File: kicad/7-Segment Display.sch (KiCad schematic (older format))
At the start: 23 parts, among them U7 74AC574, U8 74AC574, U9 74AHC02

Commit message: Working on SD card interface, cleaning up.
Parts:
- removed U7, U8: 74AC574, Housings_DIP:DIP-20_W7.62mm_LongPads, symbol 74xx:74LS574
- added U7, U8: 74AC273, symbol 74xx:74LS273
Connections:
- net labels added: ~RESET
- wire segments 77 -> 79
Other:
- moved on the sheet: R21, R22, R23, R24, R25, R26, R27, R28
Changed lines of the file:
@@
 $Descr USLetter 11000 8500
 encoding utf-8
-Sheet 3 9
+Sheet 3 10
 Title "7-Segment Display"
 Date "2018-07-20"
@@
 Comment4 ""
 $EndDescr
-$Comp
-L power:GND #PWR032
-U 1 1 59D6D694
-P 4950 4000
-F 0 "#PWR032" H 4950 3750 50  0001 C CNN
-F 1 "GND" H 4950 3850 50  0000 C CNN
-F 2 "" H 4950 4000 50  0001 C CNN
-F 3 "" H 4950 4000 50  0001 C CNN
-	1    4950 4000
-	1    0    0    -1
-$EndComp
 Entry Wire Line
 	4500 3500 4600 3400
@@
 D7
 $Comp
-L 74xx:74LS574 U7
-U 1 1 59D6D6AA
-P 5450 3200
-F 0 "U7" H 5450 3200 50  0000 C CNN
-F 1 "74AC574" H 5500 2850 50  0000 C CNN
-F 2 "Housings_DIP:DIP-20_W7.62mm_LongPads" H 5450 3200 50  0001 C CNN
-F 3 "" H 5450 3200 50  0001 C CNN
-	1    5450 3200
-	1    0    0    -1
-$EndComp
-$Comp
 L Device:R R12
 U 1 1 59D6D6B1
@@
 	0    1    1    0
 $EndComp
-$Comp
-L power:GND #PWR033
-U 1 1 59D6D6E9
-P 4950 5550
-F 0 "#PWR033" H 4950 5300 50  0001 C CNN
-F 1 "GND" H 4950 5400 50  0000 C CNN
-F 2 "" H 4950 5550 50  0001 C CNN
-F 3 "" H 4950 5550 50  0001 C CNN
-	1    4950 5550
-	1    0    0    -1
-$EndComp
+Entry Wire Line
+	4500 5550 4600 5450
+Entry Wire Line
+	4500 5450 4600 5350
 Entry Wire Line
 	4500 5350 4600 5250
@@
 Entry Wire Line
 	4500 4850 4600 4750
-Entry Wire Line
-	4500 4750 4600 4650
-Entry Wire Line
-	4500 4650 4600 4550
-Text Label 4600 4550 0    60   ~ 0
+Text Label 4600 4750 0    60   ~ 0
 D0
-Text Label 4600 4650 0    60   ~ 0
+Text Label 4600 4850 0    60   ~ 0
 D1
-Text Label 4600 4750 0    60   ~ 0
+Text Label 4600 4950 0    60   ~ 0
 D2
-Text Label 4600 4850 0    60   ~ 0
+Text Label 4600 5050 0    60   ~ 0
 D3
-Text Label 4600 4950 0    60   ~ 0
+Text Label 4600 5150 0    60   ~ 0
 D4
-Text Label 4600 5050 0    60   ~ 0
+Text Label 4600 5250 0    60   ~ 0
 D5
-Text Label 4600 5150 0    60   ~ 0
+Text Label 4600 5350 0    60   ~ 0
 D6
-Text Label 4600 5250 0    60   ~ 0
+Text Label 4600 5450 0    60   ~ 0
 D7
-$Comp
-L 74xx:74LS574 U8
-U 1 1 59D6D6FF
-P 5450 5050
-F 0 "U8" H 5450 5050 50  0000 C CNN
-F 1 "74AC574" H 5500 4700 50  0000 C CNN
-F 2 "Housings_DIP:DIP-20_W7.62mm_LongPads" H 5450 5050 50  0001 C CNN
-F 3 "" H 5450 5050 50  0001 C CNN
-	1    5450 5050
-	1    0    0    -1
-$EndComp
 $Comp
 L Device:R R21
 U 1 1 59D6D706
-P 6300 4550
-F 0 "R21" V 6261 4660 50  0000 L CNN
-F 1 "220R" V 6300 4550 50  0000 C CNN
-F 2 "Resistors_THT:R_Axial_DIN0204_L3.6mm_D1.6mm_P5.08mm_Horizontal" V 6230 4550 50  0001 C CNN
-F 3 "" H 6300 4550 50  0001 C CNN
-	1    6300 4550
-	0    1    1    0
-$EndComp
-$Comp
-L Device:R R22
-U 1 1 59D6D70D
-P 6300 4650
-F 0 "R22" V 6261 4760 50  0000 L CNN
-F 1 "220R" V 6300 4650 50  0000 C CNN
-F 2 "Resistors_THT:R_Axial_DIN0204_L3.6mm_D1.6mm_P5.08mm_Horizontal" V 6230 4650 50  0001 C CNN
-F 3 "" H 6300 4650 50  0001 C CNN
-	1    6300 4650
-	0    1    1    0
-$EndComp
-$Comp
-L Device:R R23
-U 1 1 59D6D714
 P 6300 4750
-F 0 "R23" V 6261 4860 50  0000 L CNN
+F 0 "R21" V 6261 4860 50  0000 L CNN
 F 1 "220R" V 6300 4750 50  0000 C CNN
 F 2 "Resistors_THT:R_Axial_DIN0204_L3.6mm_D1.6mm_P5.08mm_Horizontal" V 6230 4750 50  0001 C CNN
@@
 $EndComp
 $Comp
-L Device:R R24
-U 1 1 59D6D71B
+L Device:R R22
+U 1 1 59D6D70D
 P 6300 4850
-F 0 "R24" V 6261 4960 50  0000 L CNN
+F 0 "R22" V 6261 4960 50  0000 L CNN
 F 1 "220R" V 6300 4850 50  0000 C CNN
 F 2 "Resistors_THT:R_Axial_DIN0204_L3.6mm_D1.6mm_P5.08mm_Horizontal" V 6230 4850 50  0001 C CNN
@@
 $EndComp
 $Comp
-L Device:R R25
-U 1 1 59D6D722
+L Device:R R23
+U 1 1 59D6D714
 P 6300 4950
-F 0 "R25" V 6261 5060 50  0000 L CNN
+F 0 "R23" V 6261 5060 50  0000 L CNN
 F 1 "220R" V 6300 4950 50  0000 C CNN
 F 2 "Resistors_THT:R_Axial_DIN0204_L3.6mm_D1.6mm_P5.08mm_Horizontal" V 6230 4950 50  0001 C CNN
@@
 $EndComp
 $Comp
-L Device:R R26
-U 1 1 59D6D729
+L Device:R R24
+U 1 1 59D6D71B
 P 6300 5050
-F 0 "R26" V 6261 5160 50  0000 L CNN
+F 0 "R24" V 6261 5160 50  0000 L CNN
 F 1 "220R" V 6300 5050 50  0000 C CNN
 F 2 "Resistors_THT:R_Axial_DIN0204_L3.6mm_D1.6mm_P5.08mm_Horizontal" V 6230 5050 50  0001 C CNN
@@
 $EndComp
 $Comp
-L Device:R R27
-U 1 1 59D6D730
+L Device:R R25
+U 1 1 59D6D722
 P 6300 5150
-F 0 "R27" V 6261 5260 50  0000 L CNN
+F 0 "R25" V 6261 5260 50  0000 L CNN
 F 1 "220R" V 6300 5150 50  0000 C CNN
 F 2 "Resistors_THT:R_Axial_DIN0204_L3.6mm_D1.6mm_P5.08mm_Horizontal" V 6230 5150 50  0001 C CNN
@@
 $EndComp
 $Comp
-L Device:R R28
-U 1 1 59D6D737
+L Device:R R26
+U 1 1 59D6D729
 P 6300 5250
-F 0 "R28" V 6261 5360 50  0000 L CNN
+F 0 "R26" V 6261 5360 50  0000 L CNN
 F 1 "220R" V 6300 5250 50  0000 C CNN
 F 2 "Resistors_THT:R_Axial_DIN0204_L3.6mm_D1.6mm_P5.08mm_Horizontal" V 6230 5250 50  0001 C CNN
 F 3 "" H 6300 5250 50  0001 C CNN
 	1    6300 5250
+	0    1    1    0
+$EndComp
+$Comp
+L Device:R R27
+U 1 1 59D6D730
+P 6300 5350
+F 0 "R27" V 6261 5460 50  0000 L CNN
+F 1 "220R" V 6300 5350 50  0000 C CNN
+F 2 "Resistors_THT:R_Axial_DIN0204_L3.6mm_D1.6mm_P5.08mm_Horizontal" V 6230 5350 50  0001 C CNN
+F 3 "" H 6300 5350 50  0001 C CNN
+	1    6300 5350
+	0    1    1    0
+$EndComp
+$Comp
+L Device:R R28
+U 1 1 59D6D737
+P 6300 5450
+F 0 "R28" V 6261 5560 50  0000 L CNN
+F 1 "220R" V 6300 5450 50  0000 C CNN
+F 2 "Resistors_THT:R_Axial_DIN0204_L3.6mm_D1.6mm_P5.08mm_Horizontal" V 6230 5450 50  0001 C CNN
+F 3 "" H 6300 5450 50  0001 C CNN
+	1    6300 5450
 	0    1    1    0
 $EndComp
@@
 	8200 2700 8250 2700
 Wire Wire Line
-	8250 4550 6450 4550
+	8250 4750 6450 4750
 Wire Wire Line
 	8200 2800 8300 2800
 Wire Wire Line
-	8300 4650 6450 4650
+	8300 4850 6450 4850
 Wire Wire Line
 	8200 2900 8350 2900
 Wire Wire Line
-	8350 4750 6450 4750
+	8350 4950 6450 4950
 Wire Wire Line
 	8200 3000 8400 3000
 Wire Wire Line
-	8400 4850 6450 4850
+	8400 5050 6450 5050
 Wire Wire Line
 	8200 3100 8450 3100
 Wire Wire Line
-	8450 4950 6450 4950
+	8450 5150 6450 5150
 Wire Wire Line
 	8200 3200 8500 3200
 Wire Wire Line
-	8500 5050 6450 5050
+	8500 5250 6450 5250
 Wire Wire Line
 	8200 3300 8550 3300
 Wire Wire Line
-	8550 5150 6450 5150
+	8550 5350 6450 5350
 Wire Wire Line
 	8200 3400 8600 3400
 Wire Wire Line
-	8600 5250 6450 5250
+	8600 5450 6450 5450
 $Comp
 L power:GND #PWR034
@@
 Wire Wire Line
 	1450 5000 3200 5000
-Text HLabel 1450 2250 0    60   BiDi ~ 0
+Text HLabel 1450 2450 0    60   BiDi ~ 0
 D[0..7]
 Wire Bus Line
-	1450 2250 4500 2250
+	1450 2450 4500 2450
 Text HLabel 1450 3500 0    60   Input ~ 0
 ~WR
@@
 	3800 3600 4950 3600
 Wire Wire Line
-	4600 4550 4950 4550
-Wire Wire Line
-	4600 4650 4950 4650
-Wire Wire Line
 	4600 4750 4950 4750
 Wire Wire Line
@@
 	4600 5250 4950 5250
 Wire Wire Line
-	3800 5450 4950 5450
-Wire Wire Line
-	5950 4550 6150 4550
-Wire Wire Line
-	6150 4650 5950 4650
+	4600 5350 4950 5350
+Wire Wire Line
+	4600 5450 4950 5450
+Wire Wire Line
+	3800 5650 4950 5650
 Wire Wire Line
 	5950 4750 6150 4750
@@
 Wire Wire Line
 	6150 5250 5950 5250
+Wire Wire Line
+	5950 5350 6150 5350
+Wire Wire Line
+	6150 5450 5950 5450
 Wire Wire Line
 	5950 2700 6150 2700
@@
 L power:GND #PWR0108
 U 1 1 5C4980BE
-P 5450 5850
-F 0 "#PWR0108" H 5450 5600 50  0001 C CNN
-F 1 "GND" H 5455 5677 50  0000 C CNN
-F 2 "" H 5450 5850 50  0001 C CNN
-F 3 "" H 5450 5850 50  0001 C CNN
-	1    5450 5850
-	1    0    0    -1
-$EndComp
-Wire Wire Line
-	5450 4000 4950 4000
-Wire Wire Line
-	4950 4000 4950 3700
+P 5450 6050
+F 0 "#PWR0108" H 5450 5800 50  0001 C CNN
+F 1 "GND" H 5455 5877 50  0000 C CNN
+F 2 "" H 5450 6050 50  0001 C CNN
+F 3 "" H 5450 6050 50  0001 C CNN
+	1    5450 6050
+	1    0    0    -1
+$EndComp
 $Comp
 L power:VCC #PWR0109
 U 1 1 5C4A51B5
-P 5450 4250
-F 0 "#PWR0109" H 5450 4100 50  0001 C CNN
-F 1 "VCC" H 5467 4423 50  0000 C CNN
-F 2 "" H 5450 4250 50  0001 C CNN
-F 3 "" H 5450 4250 50  0001 C CNN
-	1    5450 4250
-	1    0    0    -1
-$EndComp
-Wire Wire Line
-	3800 5450 3800 4900
-Wire Wire Line
-	8250 2700 8250 4550
-Wire Wire Line
-	8300 2800 8300 4650
-Wire Wire Line
-	8350 2900 8350 4750
-Wire Wire Line
-	8400 3000 8400 4850
-Wire Wire Line
-	8450 3100 8450 4950
-Wire Wire Line
-	8500 3200 8500 5050
-Wire Wire Line
-	8550 3300 8550 5150
-Wire Wire Line
-	8600 3400 8600 5250
+P 5450 4450
+F 0 "#PWR0109" H 5450 4300 50  0001 C CNN
+F 1 "VCC" H 5467 4623 50  0000 C CNN
+F 2 "" H 5450 4450 50  0001 C CNN
+F 3 "" H 5450 4450 50  0001 C CNN
+	1    5450 4450
+	1    0    0    -1
+$EndComp
+$Comp
+L 74xx:74LS273 U7
+U 1 1 5C73DF7A
+P 5450 3200
+F 0 "U7" H 5200 3850 50  0000 C CNN
+F 1 "74AC273" H 5650 2550 50  0000 C CNN
+F 2 "" H 5450 3200 50  0001 C CNN
+F 3 "http://www.ti.com/lit/gpn/sn74LS273" H 5450 3200 50  0001 C CNN
+	1    5450 3200
+	1    0    0    -1
+$EndComp
+$Comp
+L 74xx:74LS273 U8
+U 1 1 5C74152B
+P 5450 5250
+F 0 "U8" H 5200 5900 50  0000 C CNN
+F 1 "74AC273" H 5650 4600 50  0000 C CNN
+F 2 "" H 5450 5250 50  0001 C CNN
+F 3 "http://www.ti.com/lit/gpn/sn74LS273" H 5450 5250 50  0001 C CNN
+	1    5450 5250
+	1    0    0    -1
+$EndComp
+$Comp
+L power:GND #PWR?
+U 1 1 5C74297B
+P 5450 4000
+F 0 "#PWR?" H 5450 3750 50  0001 C CNN
+F 1 "GND" H 5455 3827 50  0000 C CNN
+F 2 "" H 5450 4000 50  0001 C CNN
+F 3 "" H 5450 4000 50  0001 C CNN
+	1    5450 4000
+	1    0    0    -1
+$EndComp
+Wire Wire Line
+	3800 4900 3800 5650
+Wire Wire Line
+	8250 2700 8250 4750
+Wire Wire Line
+	8300 2800 8300 4850
+Wire Wire Line
+	8350 2900 8350 4950
+Wire Wire Line
+	8400 3000 8400 5050
+Wire Wire Line
+	8450 3100 8450 5150
+Wire Wire Line
+	8500 3200 8500 5250
+Wire Wire Line
+	8550 3300 8550 5350
+Wire Wire Line
+	8600 3400 8600 5450
+Text HLabel 1450 5750 0    60   Input ~ 0
+~RESET
+Wire Wire Line
+	1450 5750 4350 5750
+Wire Wire Line
+	4950 3700 4350 3700
+Wire Wire Line
+	4350 3700 4350 5750
 Wire Bus Line
-	4500 2250 4500 5350
-Connection ~ 4950 4000
+	4500 2450 4500 5550
+Connection ~ 4350 5750
+Wire Wire Line
+	4350 5750 4950 5750
 $EndSCHEMATC

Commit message: Assign footprints.
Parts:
- U7, U8: footprint (none) -> Housings_SSOP:TSSOP-20_4.4x6.5mm_Pitch0.65mm
- U9: footprint Housings_DIP:DIP-14_W7.62mm_LongPads -> Housings_DIP:DIP-14_W7.62mm
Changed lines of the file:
@@
 F 0 "U9" H 3500 3650 50  0000 C CNN
 F 1 "74AHC02" H 3550 3550 50  0000 C CNN
-F 2 "Housings_DIP:DIP-14_W7.62mm_LongPads" H 3500 3600 50  0001 C CNN
+F 2 "Housings_DIP:DIP-14_W7.62mm" H 3500 3600 50  0001 C CNN
 F 3 "" H 3500 3600 50  0001 C CNN
 	1    3500 3600
@@
 F 0 "U9" H 3500 4950 50  0000 C CNN
 F 1 "74AHC02" H 3550 4850 50  0000 C CNN
-F 2 "Housings_DIP:DIP-14_W7.62mm_LongPads" H 3500 4900 50  0001 C CNN
+F 2 "Housings_DIP:DIP-14_W7.62mm" H 3500 4900 50  0001 C CNN
 F 3 "" H 3500 4900 50  0001 C CNN
 	2    3500 4900
@@
 F 0 "U7" H 5200 3850 50  0000 C CNN
 F 1 "74AC273" H 5650 2550 50  0000 C CNN
-F 2 "" H 5450 3200 50  0001 C CNN
+F 2 "Housings_SSOP:TSSOP-20_4.4x6.5mm_Pitch0.65mm" H 5450 3200 50  0001 C CNN
 F 3 "http://www.ti.com/lit/gpn/sn74LS273" H 5450 3200 50  0001 C CNN
 	1    5450 3200
@@
 F 0 "U8" H 5200 5900 50  0000 C CNN
 F 1 "74AC273" H 5650 4600 50  0000 C CNN
-F 2 "" H 5450 5250 50  0001 C CNN
+F 2 "Housings_SSOP:TSSOP-20_4.4x6.5mm_Pitch0.65mm" H 5450 5250 50  0001 C CNN
 F 3 "http://www.ti.com/lit/gpn/sn74LS273" H 5450 5250 50  0001 C CNN
 	1    5450 5250

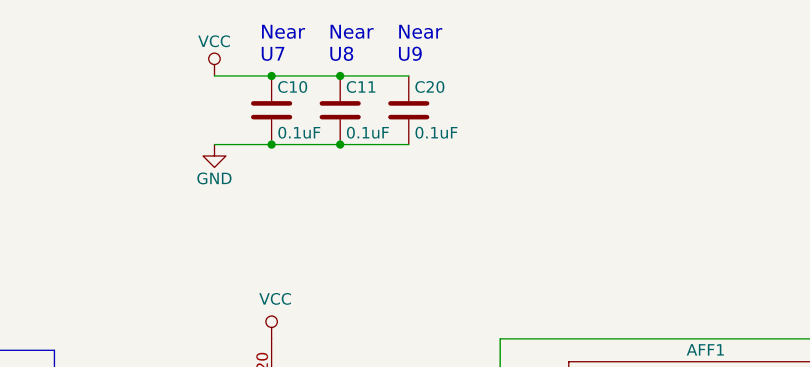
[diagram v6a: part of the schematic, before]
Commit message: First pass layout of revised board complete.
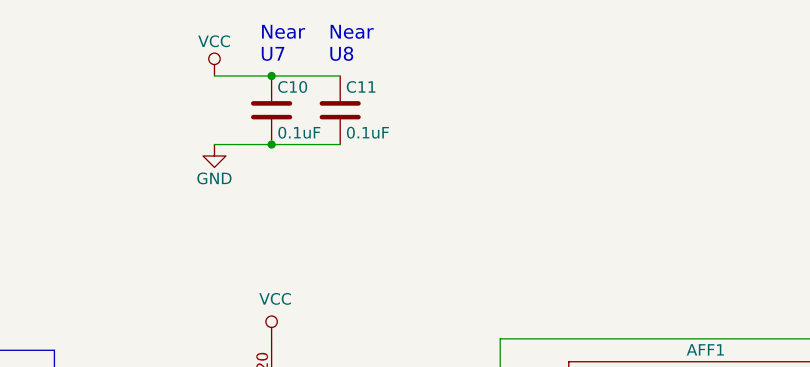
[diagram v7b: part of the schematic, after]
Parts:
- removed C20: 0.1uF, Capacitors_THT:C_Disc_D4.3mm_W1.9mm_P5.00mm, symbol Device:C
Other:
- note removed: "Near\nU9"
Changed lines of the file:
@@
 Sheet 3 11
 Title "7-Segment Display"
-Date "2019-04-11"
+Date "2019-04-15"
 Rev "1"
 Comp ""
@@
 Connection ~ 5450 1250
 Connection ~ 5450 1550
-Connection ~ 5750 1250
-Connection ~ 5750 1550
 Wire Wire Line
 	5200 1550 5450 1550
@@
 	1    0    0    -1
 $EndComp
-$Comp
-L Device:C C20
-U 1 1 59EFD5EA
-P 6050 1400
-F 0 "C20" H 6075 1500 50  0000 L CNN
-F 1 "0.1uF" H 6075 1300 50  0000 L CNN
-F 2 "Capacitors_THT:C_Disc_D4.3mm_W1.9mm_P5.00mm" H 6088 1250 50  0001 C CNN
-F 3 "" H 6050 1400 50  0001 C CNN
-	1    6050 1400
-	1    0    0    -1
-$EndComp
-Text Notes 6000 1200 0    60   ~ 0
-Near\nU9
 Wire Wire Line
 	2050 3500 3200 3500
@@
 	5450 1550 5750 1550
 Wire Wire Line
-	5750 1250 6050 1250
-Wire Wire Line
-	5750 1550 6050 1550
-Wire Wire Line
 	4600 2700 4950 2700
